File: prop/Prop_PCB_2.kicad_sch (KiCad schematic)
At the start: 42 parts

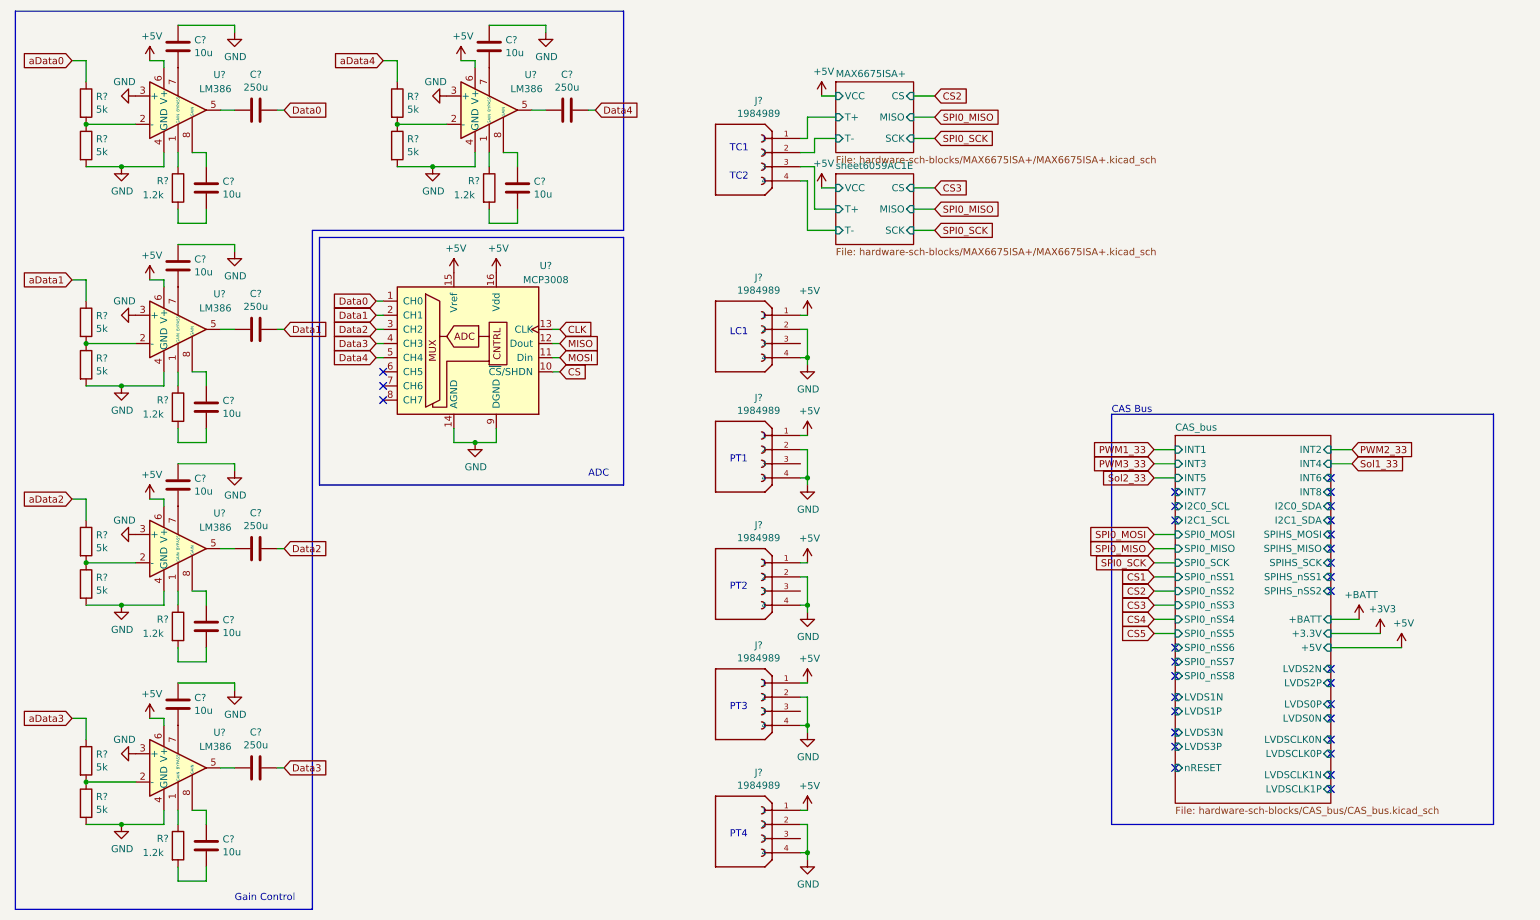
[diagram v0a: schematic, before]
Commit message: finalize3pcb schematic
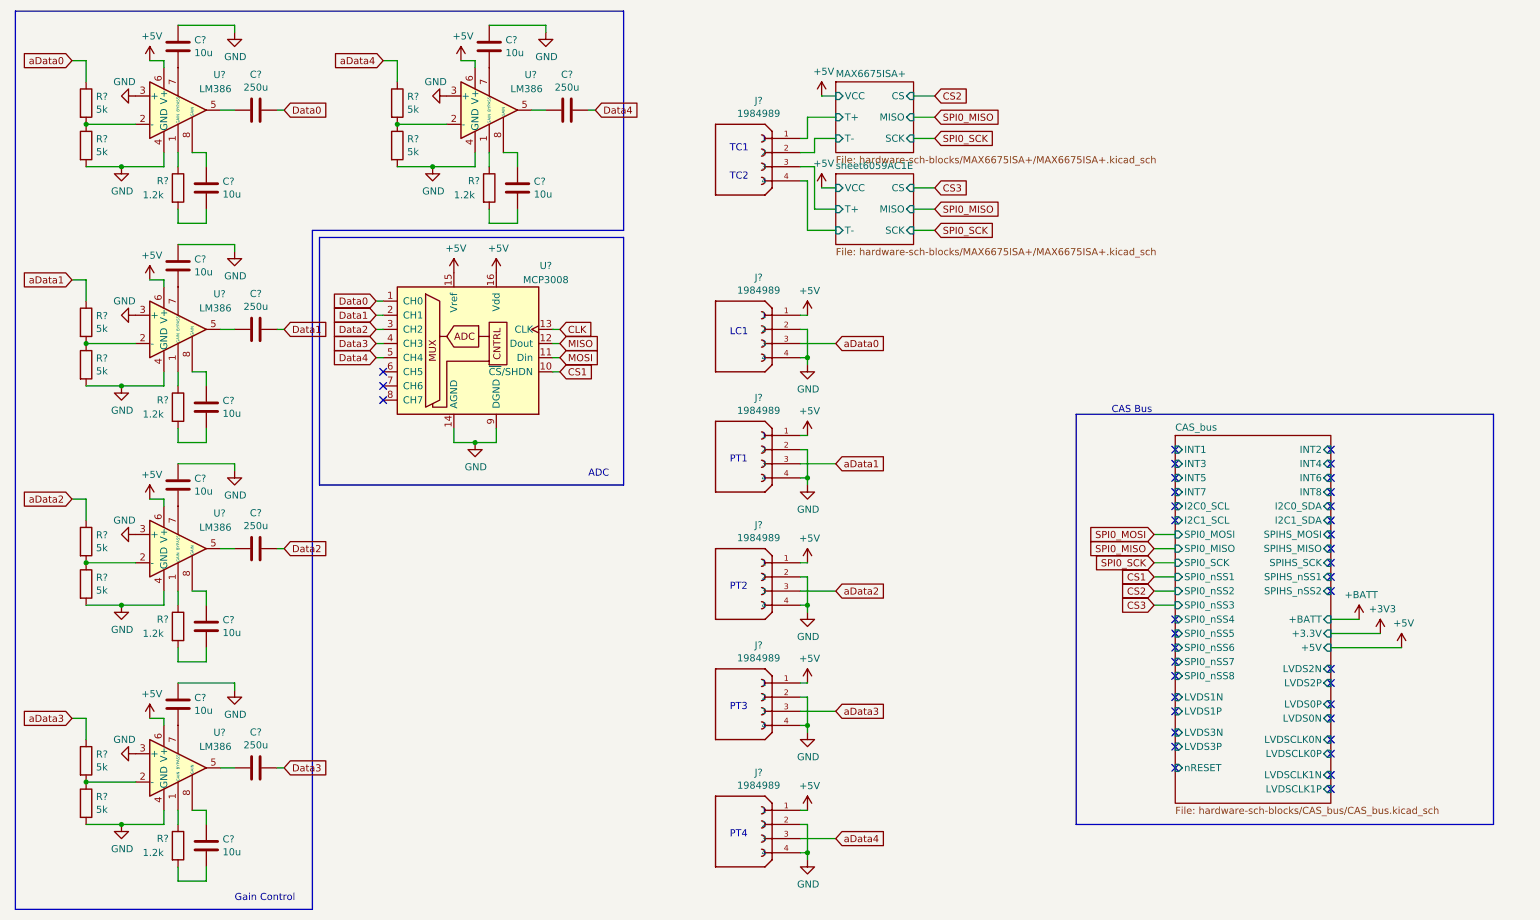
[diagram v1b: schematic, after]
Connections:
- net CS is gone; now on net CS1: U?.10 (~{CS}/SHDN)
- net aData0: now also J?.3
- net aData1: now also J?.3
- net aData2: now also J?.3
- net aData3: now also J?.3
- net aData4: now also J?.3
- no-connect marks 31 -> 38
